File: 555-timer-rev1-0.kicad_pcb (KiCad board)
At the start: 2 copper layers, 13.5 x 35.2 mm, 19 parts, among them J1 Conn_01x02_Male, SW1 SW_Push, SW2 SW_Push, U1 SA555D

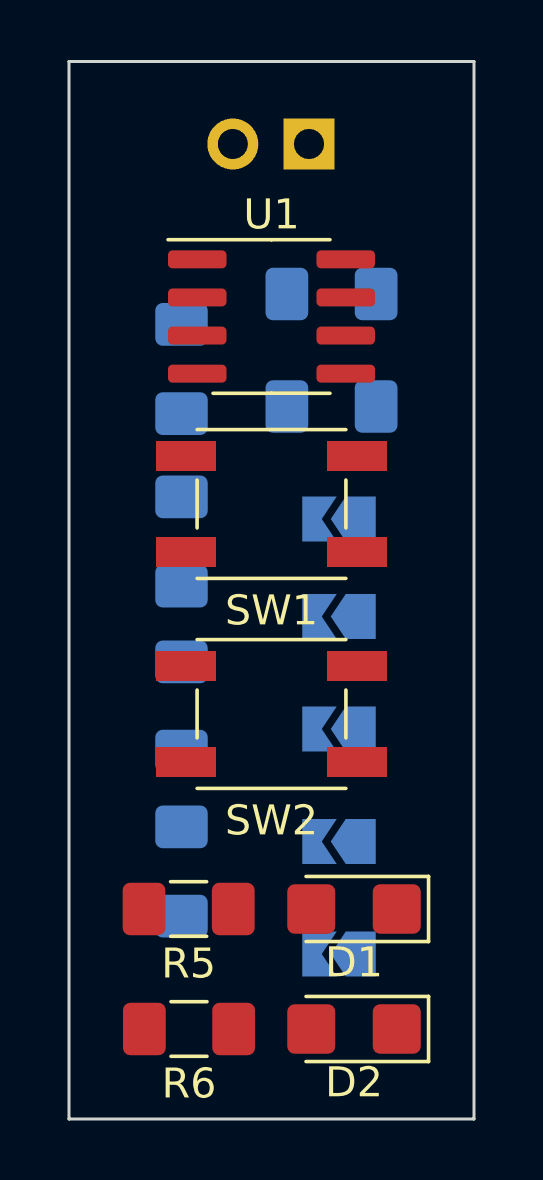
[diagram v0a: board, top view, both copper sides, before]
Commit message: Finish PCB layout.
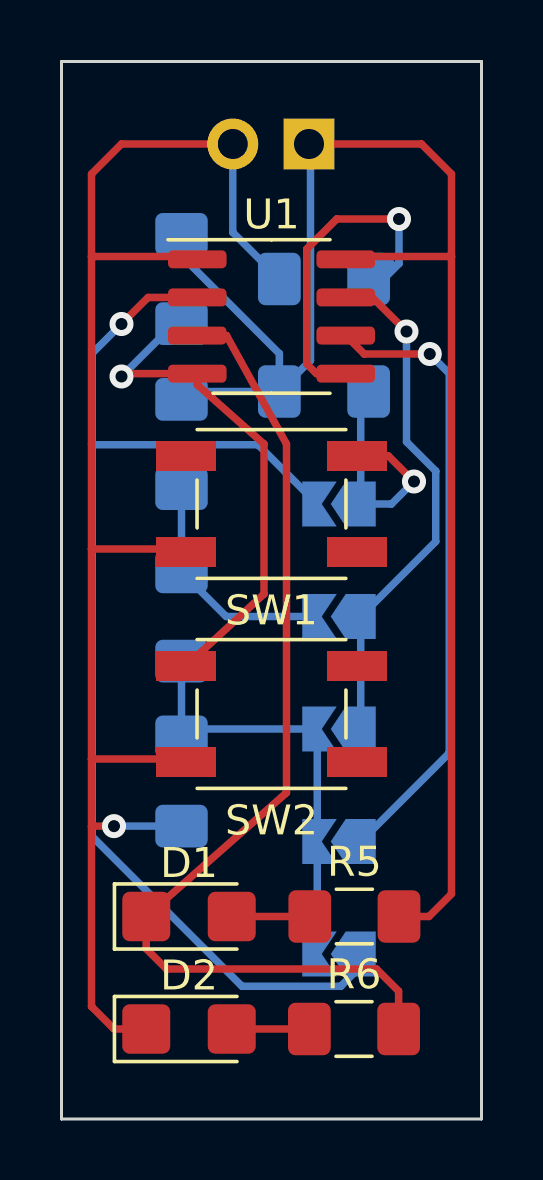
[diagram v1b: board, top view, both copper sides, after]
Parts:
- moved C1 20.3 mm to (150.5, 79.5), turned to 180 degrees
- moved R2 6.56 mm to (145.8, 79.5), turned to 270 degrees
- moved R5 5.53 mm to (151.5, 100.8), turned to 0 degrees
- moved D1 5.51 mm to (146.0, 100.8), turned to 0 degrees
- moved D2 5.50 mm to (146.0, 104.5), turned to 0 degrees
- moved R6 5.50 mm to (151.5, 104.5), turned to 0 degrees
- moved R1 3.26 mm to (150.5, 83.2)
- moved C2 2.50 mm to (145.8, 96.2)
- moved R3 2.50 mm to (145.8, 85.0)
- moved R4 2.50 mm to (145.8, 90.8)
- moved JP1 0.50 mm to (151.0, 87.0)
- renumbered JP3 to JP2, JP4 to JP3, JP5 to JP4, JP2 to JP5
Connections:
- C2 pad 1: /TRIGGER -> Net-(C2-Pad1)
- JP1 pad 2: Net-(JP1-Pad2) -> /TRIGGER
- JP3 pad 2: /TRIGGER -> Net-(C2-Pad1)
- JP4 pad 2: /TRIGGER -> Net-(C2-Pad1)
- JP5 pad 1: Net-(JP1-Pad1) -> /TRIGGER
- JP5 pad 2: /TRIGGER -> Net-(C2-Pad1)
- R1 pad 1: +5V -> Net-(JP1-Pad1)
- R1 pad 2: Net-(JP1-Pad2) -> +5V
- R4 pad 2: /TRIGGER -> Net-(C2-Pad1)
- R5 pad 1: +5V -> Net-(D1-Pad2)
- R5 pad 2: Net-(D1-Pad2) -> +5V
- R6 pad 1: Net-(D1-Pad1) -> Net-(D2-Pad2)
- R6 pad 2: Net-(D2-Pad2) -> Net-(D1-Pad1)
- SW1 pad 2: Net-(JP1-Pad2) -> Net-(JP1-Pad1)
- U1 pad 2: Net-(JP1-Pad1) -> /TRIGGER
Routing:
- net +5V: track 0.00 -> 54.3 mm
- net GND: track 0.00 -> 53.1 mm, vias 0 -> 1
- net /TRIGGER: track 0.00 -> 40.4 mm, vias 0 -> 1
- net Net-(D1-Pad1): track 0.00 -> 34.3 mm
- net Net-(JP4-Pad1): track 0.00 -> 20.8 mm, vias 0 -> 1
- net Net-(JP2-Pad1): track 0.00 -> 17.2 mm, vias 0 -> 1
- net Net-(R2-Pad2): track 0.00 -> 17.2 mm, vias 0 -> 1
- net Net-(C2-Pad1): track 0.00 -> 14.7 mm
- net Net-(C1-Pad1): track 0.00 -> 11.3 mm, vias 0 -> 1
- net Net-(JP1-Pad1): track 0.00 -> 8.40 mm, vias 0 -> 1
- net Net-(JP2-Pad2): track 0.00 -> 7.92 mm
- net Net-(D1-Pad2): track 0.00 -> 2.60 mm
- net Net-(D2-Pad2): track 0.00 -> 2.59 mm
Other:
- board size 13.5 x 35.2 mm -> 14 x 35.2 mm
